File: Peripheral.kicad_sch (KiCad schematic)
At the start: 26 parts, among them J2 Conn_02x05_Odd_Even, J3 Conn_02x08_Odd_Even, J4 Conn_02x08_Odd_Even, J6 Bus_ISA_8bit, J7 Conn_02x17_Odd_Even, J8 TTL UART, U25 SN74LS07N, U3 74164, U31 TXS0104ED, U32 16550, U33 WD37C65, U6 74164, U9 ATF1508AS-10JU84, Y2 9.6 MHz, Y3 16 MHz

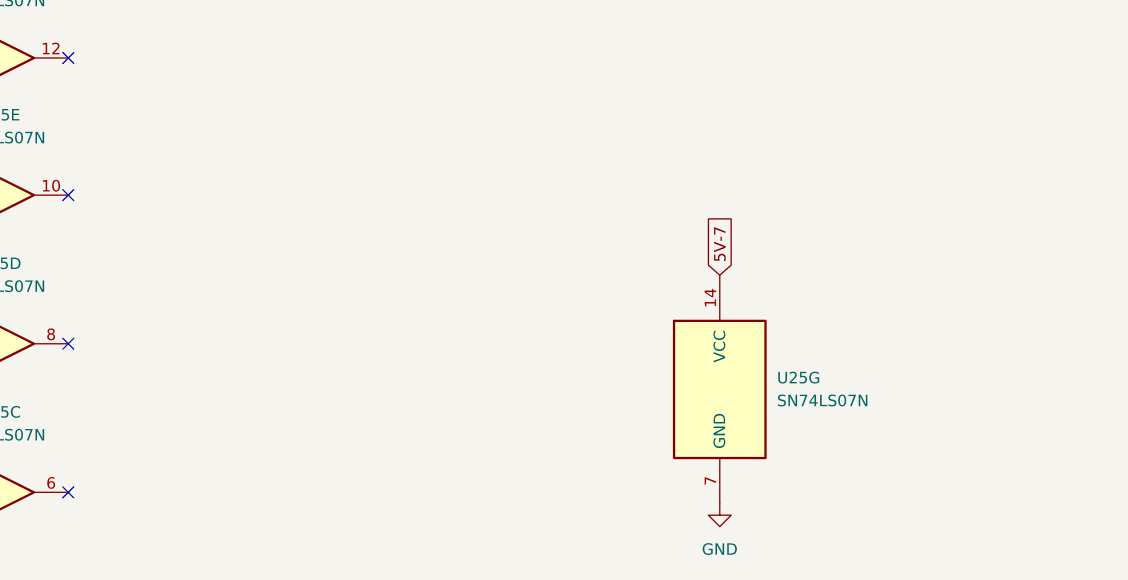
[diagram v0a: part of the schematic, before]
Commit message: Updated PCB
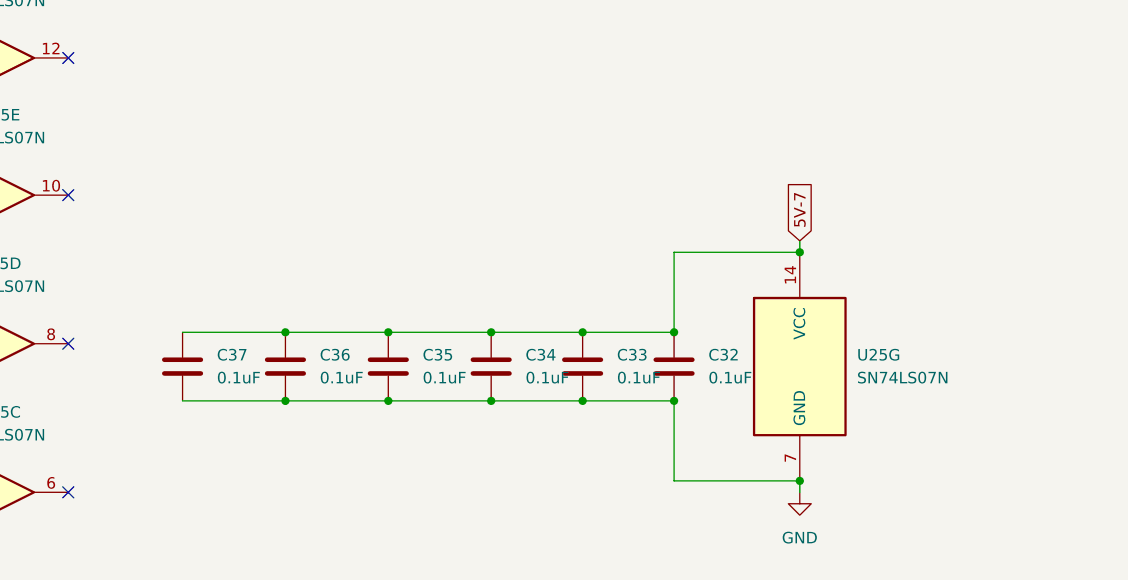
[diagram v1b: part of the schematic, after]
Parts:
- added C32, C33, C34, C35, C36, C37: 0.1uF, Capacitor_THT:C_Disc_D8.0mm_W2.5mm_P5.00mm, symbol Device:C
- U9: footprint Package_LCC:PLCC-84_29.3x29.3mm_P1.27mm -> Package_LCC:PLCC-84_THT-Socket
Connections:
- net GND: now also C32.2, C33.2, C34.2, C35.2, C36.2, C37.2
- net VCC: now also C32.1, C33.1, C34.1, C35.1, C36.1, C37.1
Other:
- moved on the sheet: U25G
